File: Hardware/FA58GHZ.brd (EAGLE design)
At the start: 41.9 x 24.1 mm, 51 parts, among them IC1 MAX4311EEE, IC2 MCP6001, IC3 MCP6001, Q2 pchanel, Q3 200mA/50V, U1 ATMEGA328P_TQFP, U2 RX5808, X1 SMA-SMDPCB, Y1 16MHZ

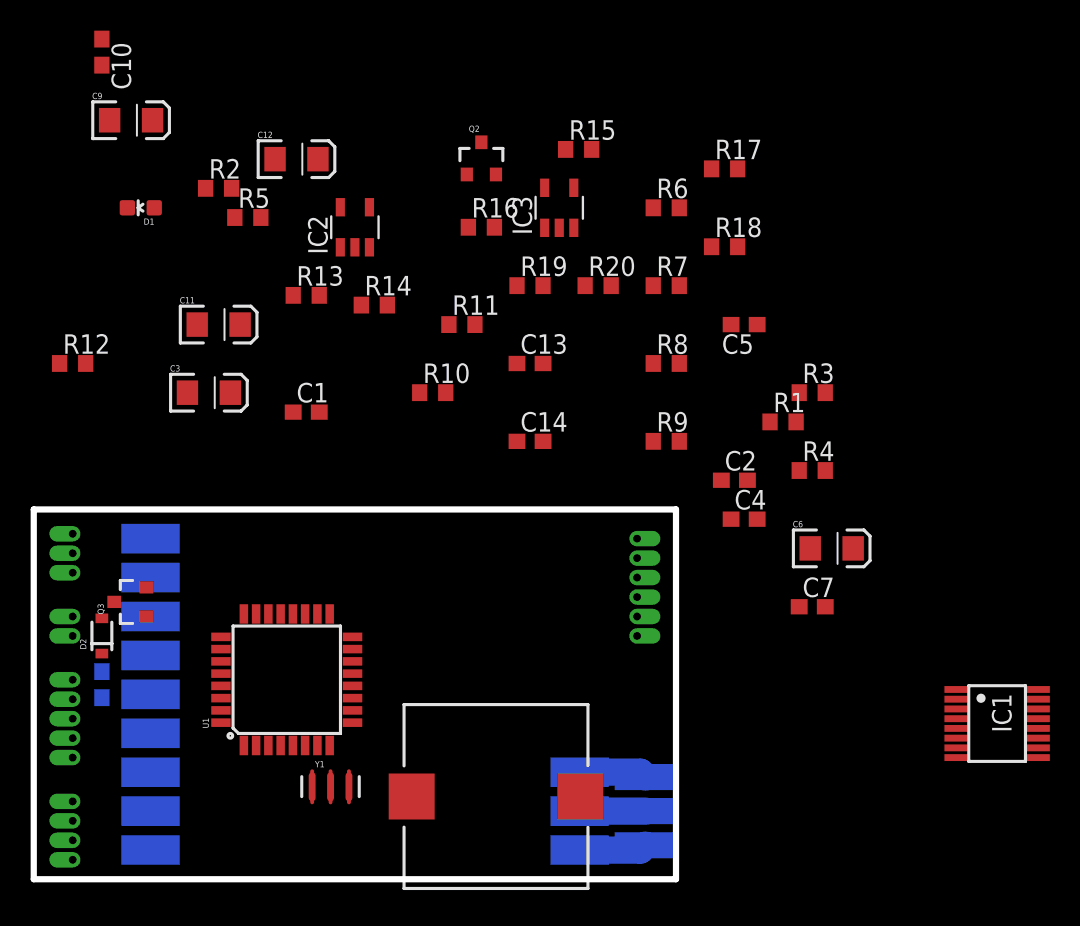
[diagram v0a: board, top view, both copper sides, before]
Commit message: Backup: PCB routing finished, need to run DRC
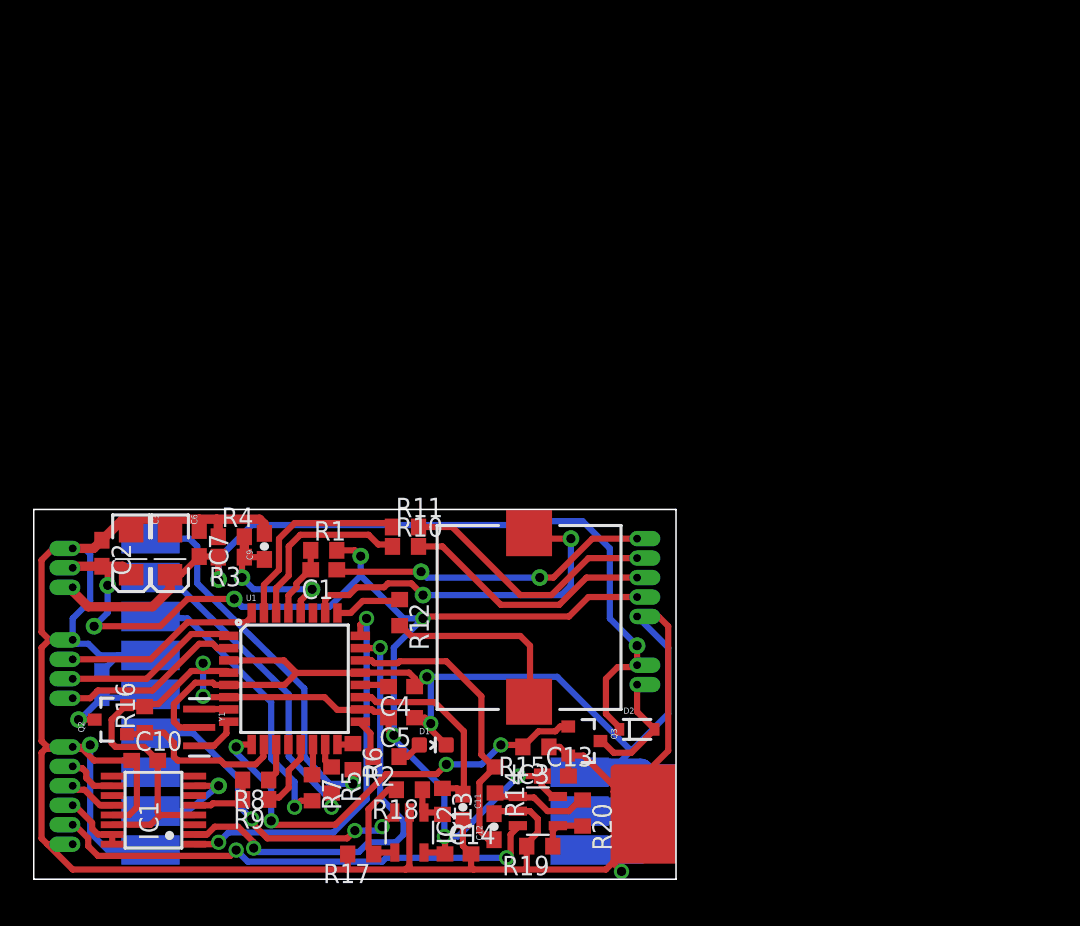
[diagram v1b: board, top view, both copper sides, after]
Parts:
- C11, C12, C9: device SparkFun-Capacitors:EIA3216 -> SparkFun-Passives:0603-CAP
- Y1: device SparkFun-FreqCtrl:RESONATOR-SMD -> FreakyAttic-EagleLibrary:RESONATOR-SMD
- moved IC1 55.3 mm to (7.81, 4.51), turned to 90 degrees
- moved R17 50.6 mm to (21.3, 1.65), turned to 180 degrees
- moved C10 46.3 mm to (7.24, 7.75), turned to 0 degrees
- moved C12 45.4 mm to (30.0, 3.43), turned to 90 degrees
- moved Q2 43.8 mm to (5.08, 10.4), turned to 90 degrees
- moved C6 43.2 mm to (8.89, 21.3), turned to 270 degrees
- moved C2 41.5 mm to (4.45, 21.3), turned to 270 degrees
- moved R6 41.2 mm to (20.8, 8.00), turned to 270 degrees
- moved R18 41.0 mm to (24.5, 5.84), turned to 180 degrees
- moved C7 40.2 mm to (10.8, 21.9), turned to 270 degrees
- moved R7 40.1 mm to (18.2, 5.97), turned to 270 degrees
- moved D1 39.9 mm to (26.0, 8.76), turned to 270 degrees
- moved IC2 39.7 mm to (24.5, 3.05), turned to 180 degrees
- moved R3 39.4 mm to (12.9, 21.0), turned to 180 degrees
- moved IC3 39.4 mm to (32.9, 4.45), turned to 270 degrees
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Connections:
- removed net +5V: JP1.2
- net AN_VPOW: now also C9.1; no longer C9.A
- net BUT1: now also JP5.2; no longer JP5.4
- net BUT3: now also JP5.4; no longer JP5.2
- net GND: now also C11.2, C12.2, C9.2; no longer C11.C, C12.C, C9.C
- net N$17: now also C12.1; no longer C12.A
- net N$18: now also C11.1; no longer C11.A
- net RSSI2: now also JP3.5; no longer JP3.4
- net VCC: now also JP1.2
- net VIDEO2: now also JP3.2; no longer JP3.3
- net VIDEO3: now also JP3.3; no longer JP3.2
- net VIDEO_OUT: now also JP3.4; no longer JP3.5
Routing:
- net GND: track 8.84 -> 236.3 mm, vias 0 -> 4
- net VCC: track 0.00 -> 120.6 mm, vias 0 -> 10
- net +12V: track 0.00 -> 56.7 mm, vias 0 -> 2
- net RSSI2: track 0.00 -> 32.6 mm, vias 0 -> 2
- net SEL0: track 0.00 -> 29.4 mm, vias 0 -> 2
- net FAN: track 0.00 -> 29.1 mm, vias 0 -> 4
- net SEL1: track 0.00 -> 25.6 mm, vias 0 -> 2
- net CLOCK: track 0.00 -> 24.8 mm, vias 0 -> 1
- net N$11: track 0.00 -> 23.9 mm, vias 0 -> 2
- net SELECT: track 0.00 -> 21.6 mm, vias 0 -> 1
- net RSSI1: track 0.00 -> 21.0 mm, vias 0 -> 3
- net DTR: track 0.00 -> 20.9 mm, vias 0 -> 2
- net N$17: track 0.00 -> 19.8 mm
- net DATA: track 0.00 -> 18.9 mm, vias 0 -> 1
- net TX: track 0.00 -> 17.1 mm
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
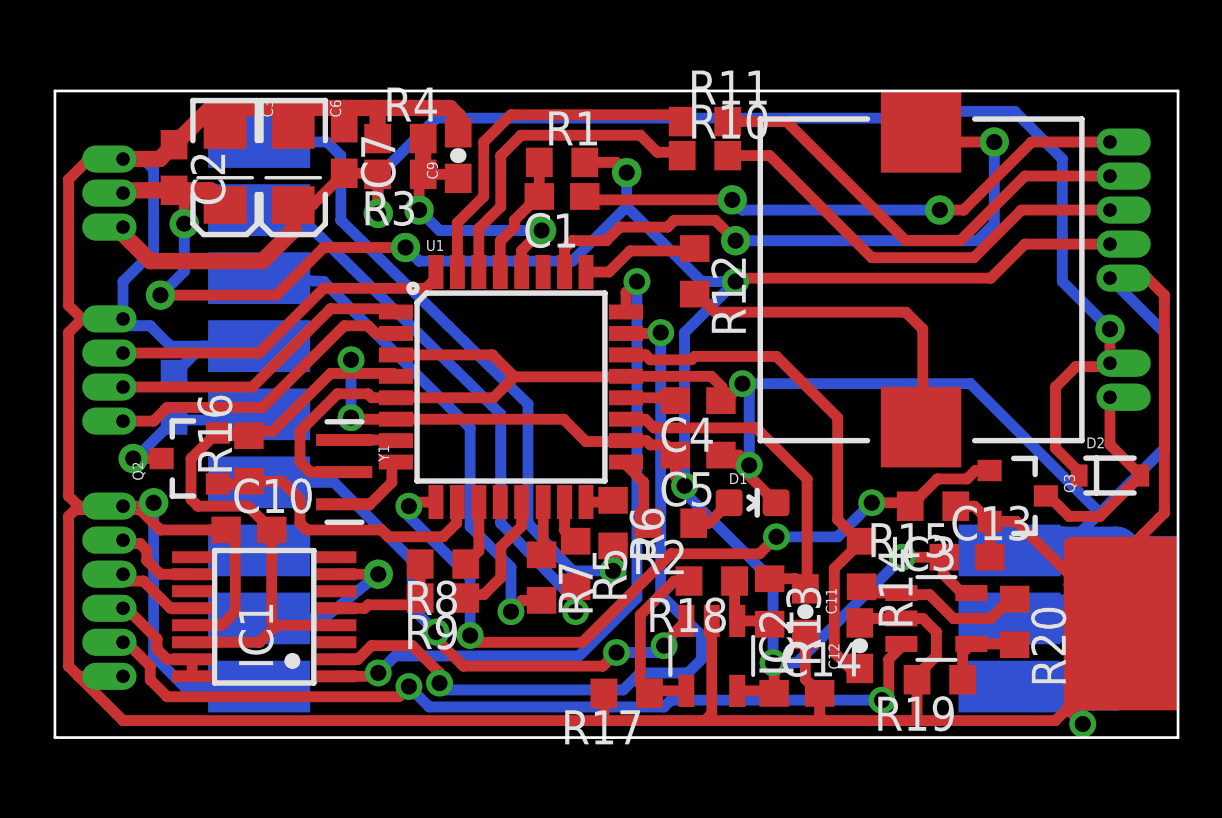
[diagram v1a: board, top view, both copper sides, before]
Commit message: -Routing finished and DRC passed with approved warnings
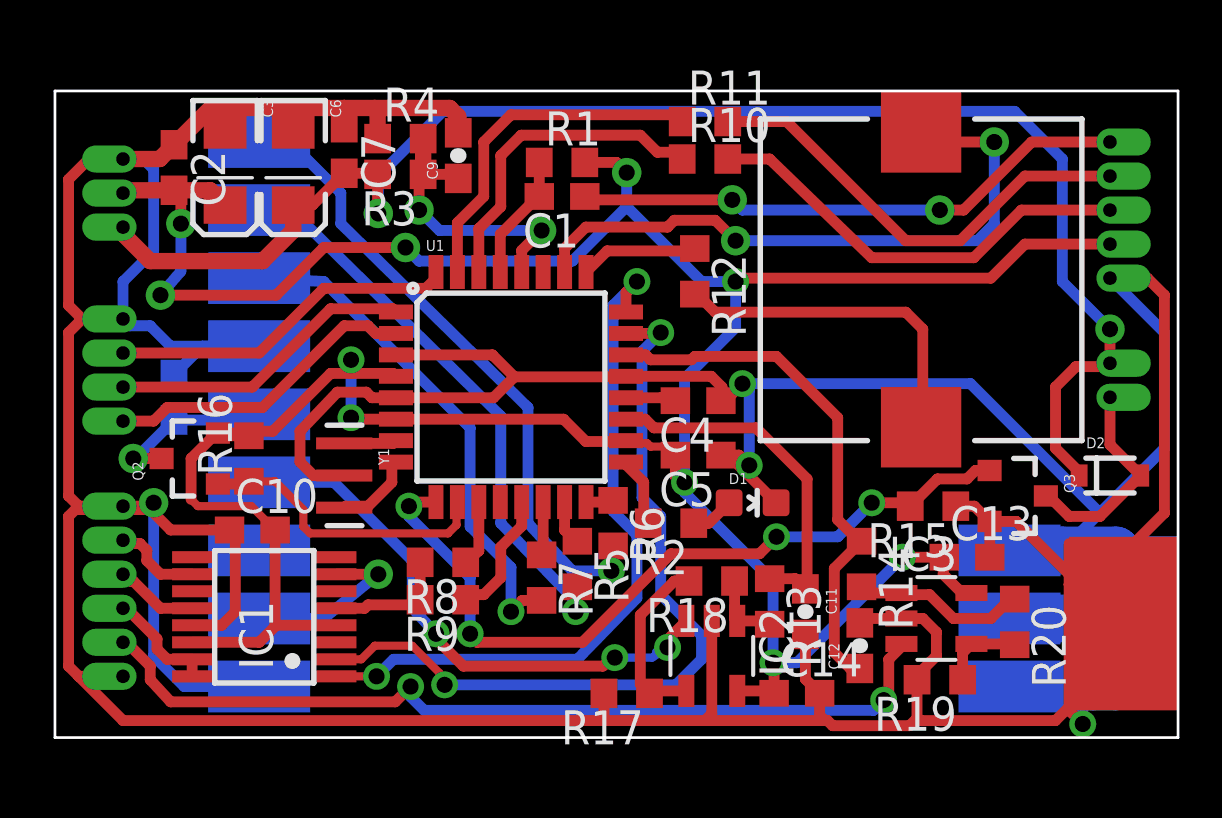
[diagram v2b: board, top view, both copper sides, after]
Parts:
- moved Y1 0.13 mm to (10.8, 9.78)
- moved C10 0.13 mm to (7.37, 7.75)
- moved R10 0.13 mm to (24.3, 21.6)
- moved R8 0.06 mm to (14.5, 6.54)
- moved R9 0.06 mm to (14.5, 5.14)
- moved R5 0.06 mm to (19.5, 6.48)
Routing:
- net CLOCK: track 24.8 -> 23.9 mm
- net SEL1: track 25.6 -> 26.4 mm
- net RSSI1: track 21.0 -> 21.5 mm
- net RSSI2: track 32.6 -> 33.1 mm
